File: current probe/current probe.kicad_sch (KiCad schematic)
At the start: 4 parts, among them U1 OPA2134

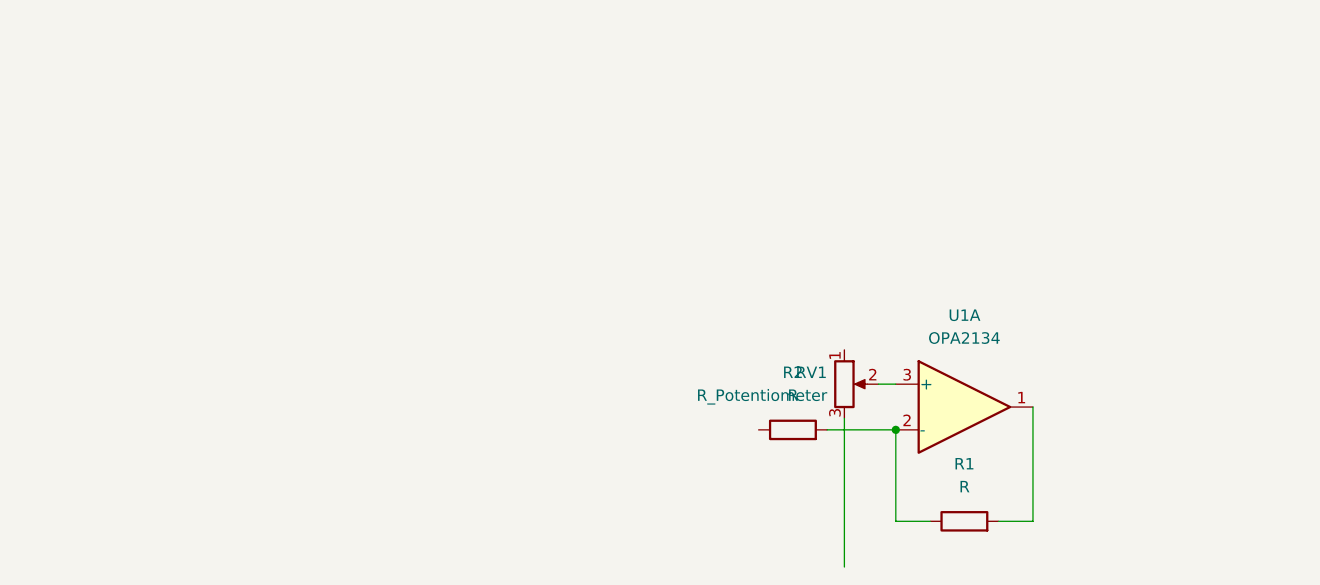
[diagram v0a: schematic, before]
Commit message: Updated schematic
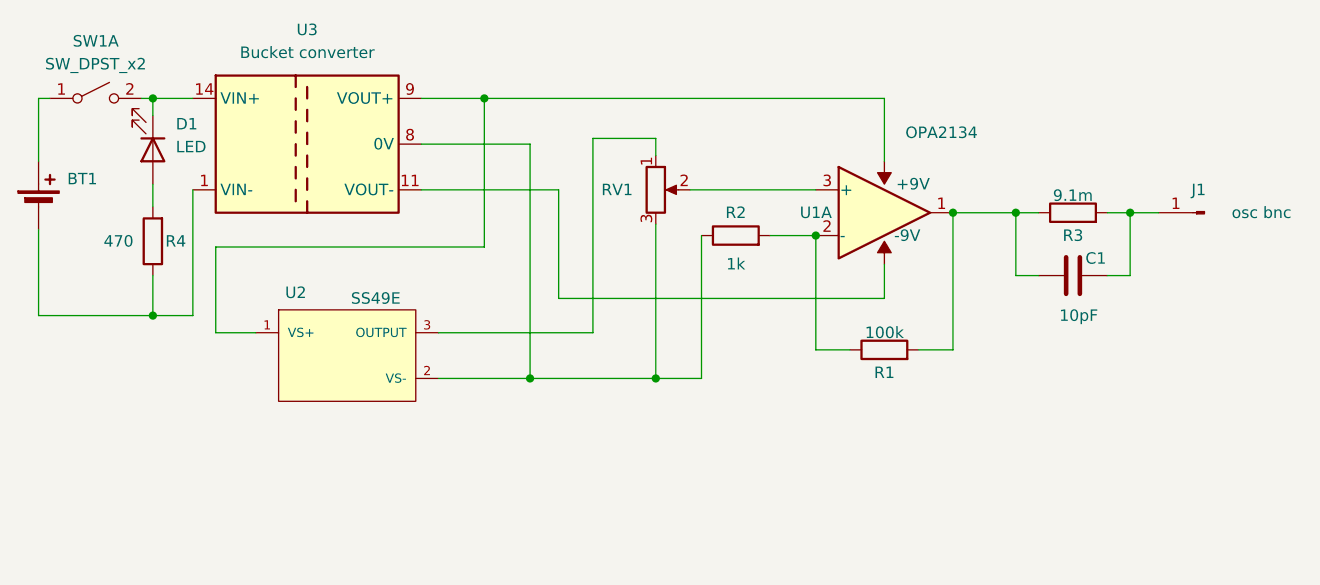
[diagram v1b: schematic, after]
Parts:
- added BT1: Battery_Cell, symbol Library:Battery_Cell
- added C1: 10pF, symbol Device:C
- added D1: LED, symbol Device:LED
- added J1: osc bnc, symbol Library:Conn_01x01_Pin
- added R3: 9.1m, symbol Library:R
- added R4: 470, symbol Library:R
- added SW1: SW_DPST_x2, symbol Library:SW_DPST_x2
- added U2: SS49E, Honeywell-SS49E-*, symbol Library:SS49E
- added U3: Bucket converter, Converter_DCDC:Converter_DCDC_Murata_NMAxxxxDC_THT, symbol Library:NMA1512DC
- R1: value R -> 100k; symbol Device:R -> Library:R
- R2: value R -> 1k; symbol Device:R -> Library:R
- RV1: symbol Device:R_Potentiometer -> Library:R_Potentiometer
- U1: symbol Amplifier_Operational:OPA2134 -> Library:OPA2134
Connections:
- net at R1.2, U1.1: now also C1.1, R3.1
- net at RV1.1: now also U2.3 (OUTPUT)
- net at RV1.3: now also R2.1, U2.2 (VS-), U3.8 (0V)
- new net: BT1.2 (-), R4.1, U3.1 (VIN-)
- new net: D1.2 (A), R4.2
- new net: C1.2, J1.1 (Pin_1), R3.2
- new net: D1.1 (K), SW1.2 (B), U3.14 (VIN+)
- new net: BT1.1 (+), SW1.1 (A)
- new net +9V: U2.1 (VS+), U3.9 (VOUT+)
- new net -9V: U3.11 (VOUT-)
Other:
- company: (none) -> YR-Design
- title: (none) -> Current probe board
- moved on the sheet: R1, R2, RV1, U1A
